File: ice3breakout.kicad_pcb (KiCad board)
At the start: 2 copper layers, 50 x 50 mm, 18 parts, among them CON1 AVR-ISP-6, CON2 AVR-JTAG-10, CON3 AVR-PDI-6, CON4 USB-MICRO-B, P1 Jtag ICE3, P2 Cortex M0 debug, P3 ice3 expansion, P4 Supply select, P5 Supply, P6 GND, SW1 SW_PUSH, U1 AP1117D33, U2 AP1117D18

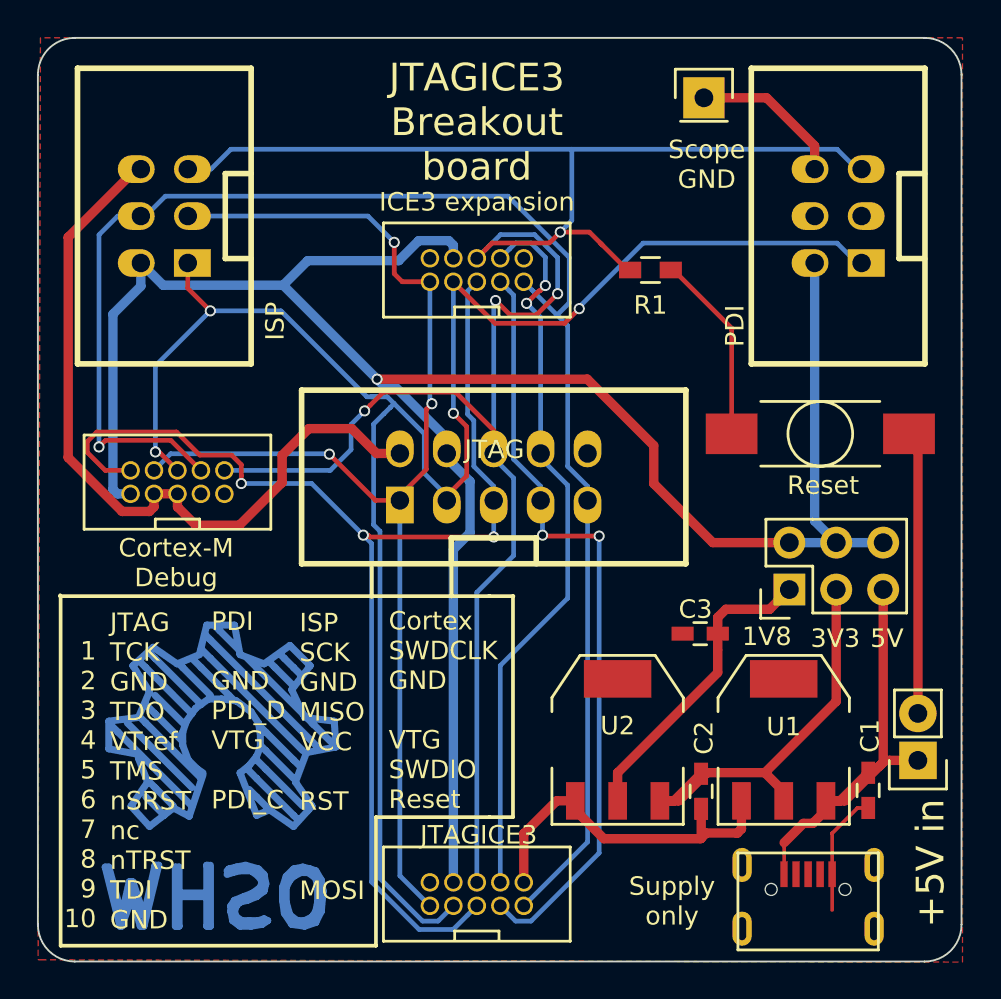
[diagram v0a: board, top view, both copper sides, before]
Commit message: closes #1, closes #2, closes #3
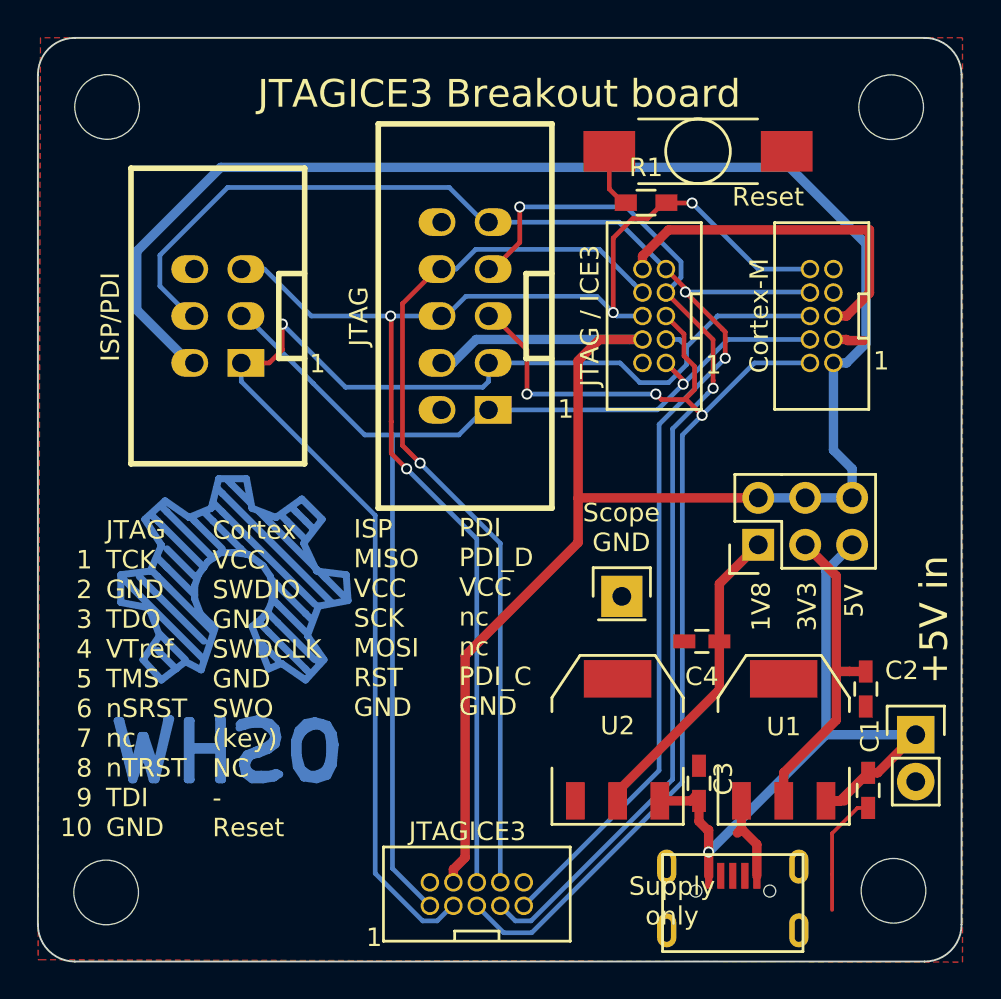
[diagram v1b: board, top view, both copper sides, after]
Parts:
- removed CON3: AVR-PDI-6, w_conn_strip:vasch_strip_3x2
- added C4: C, Capacitors_SMD:C_0603_HandSoldering, F.Cu at (139.9, 111.7)
- added REF**: MountingHole_3-5mm, Mounting_Holes:MountingHole_3-5mm, F.Cu at (150.2, 82.8)
- added REF**: MountingHole_3-5mm, Mounting_Holes:MountingHole_3-5mm, F.Cu at (107.7, 82.7)
- added REF**: MountingHole_3-5mm, Mounting_Holes:MountingHole_3-5mm, F.Cu at (107.7, 125.3)
- added REF**: MountingHole_3-5mm, Mounting_Holes:MountingHole_3-5mm, F.Cu at (150.3, 125.2)
- moved P2 36.0 mm to (146.4, 94.1), turned to 90 degrees
- moved P6 27.4 mm to (135.6, 109.2)
- moved SW1 16.7 mm to (139.7, 85.1)
- moved C2 10.5 mm to (148.8, 114.2)
- moved P3 9.92 mm to (137.4, 94.1), turned to 90 degrees
- moved CON2 8.85 mm to (127.1, 94.1), turned to 90 degrees
- moved C3 8.10 mm to (139.8, 119.4), turned to 90 degrees
- moved REF** 7.95 mm to (114.5, 89.7)
- moved CON1 6.14 mm to (113.7, 94.1)
- moved CON4 4.08 mm to (141.6, 128.5)
- moved R1 3.66 mm to (136.9, 87.9), turned to 0 degrees
- moved P4 2.95 mm to (143.0, 106.4)
- moved P5 1.39 mm to (151.5, 116.7), turned to 0 degrees
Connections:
- C3 pad 1: +1V8 -> +5V
- U2 pad 3: +3V3 -> +5V
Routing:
- net GND: track 92.0 -> 32.5 mm
- net /RST: track 115.6 -> 73.3 mm
- net Net-(CON1-Pad1): track 102.0 -> 75.1 mm, vias 4 -> 1
- net +5V: track 23.7 -> 39.1 mm, vias 0 -> 1
- net Net-(CON2-Pad7): track 42.1 -> 57.3 mm
- net Net-(CON2-Pad8): track 39.8 -> 48.7 mm, vias 2 -> 1
- net VCC: track 118.3 -> 127.1 mm, vias 1 -> 0
- net Net-(R1-Pad1): track 10.3 -> 3.23 mm
- net Net-(CON2-Pad5): track 69.4 -> 63.0 mm
- net +3V3: track 22.6 -> 17.8 mm
- net Net-(CON1-Pad4): track 85.6 -> 82.0 mm, vias 1 -> 2
- net Net-(CON1-Pad3): track 65.5 -> 63.5 mm, vias 3 -> 1
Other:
- net class Default: clearance 0.2 -> 0.1905
- net class Power: clearance 0.2 -> 0.1905
- rule trace_clearance: 0.2 -> 0.1905
- board text added: "1"
- board text added: "Cortex VCC SWDIO GND SWDCLK GND SWO (key) NC - Reset"
- board text added: "Cortex-M"
- board text added: "ISP MISO VCC SCK MOSI RST GND"
- board text added: "ISP/PDI"
- board text added: "JTAG / ICE3"
- board text added: "PDI PDI_D VCC nc nc PDI_C GND"
- board text removed: "Cortex SWDCLK GND VTG SWDIO Reset"
- board text removed: "Cortex-M Debug"
- board text removed: "ICE3 expansion"
- board text removed: "ISP"
- board text removed: "ISP SCK GND MISO VCC RST MOSI"
- board text removed: "PDI"
- board text removed: "PDI GND PDI_D VTG PDI_C"
